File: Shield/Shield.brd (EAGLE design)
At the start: 100 x 80 mm, 11 parts, among them Q1 NPN, U1 TEMPERATURE-SENSOR

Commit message: fixed D2 pin
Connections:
- removed net D2: JP4.1
- net LED: now also JP4.1
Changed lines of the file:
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@@
 </elements>
 <signals>
-<signal name="D2">
-<contactref element="JP4" pad="1"/>
-</signal>
 <signal name="MST">
 <contactref element="YUN1" pad="A0"/>
@@
 <signal name="LED">
 <contactref element="YUN1" pad="D2"/>
+<contactref element="JP4" pad="1"/>
+<wire x1="53.312078125" y1="24.739640625" x2="26.27139375" y2="67.21223125" width="0" layer="19" extent="1-1"/>
 </signal>
 </signals>

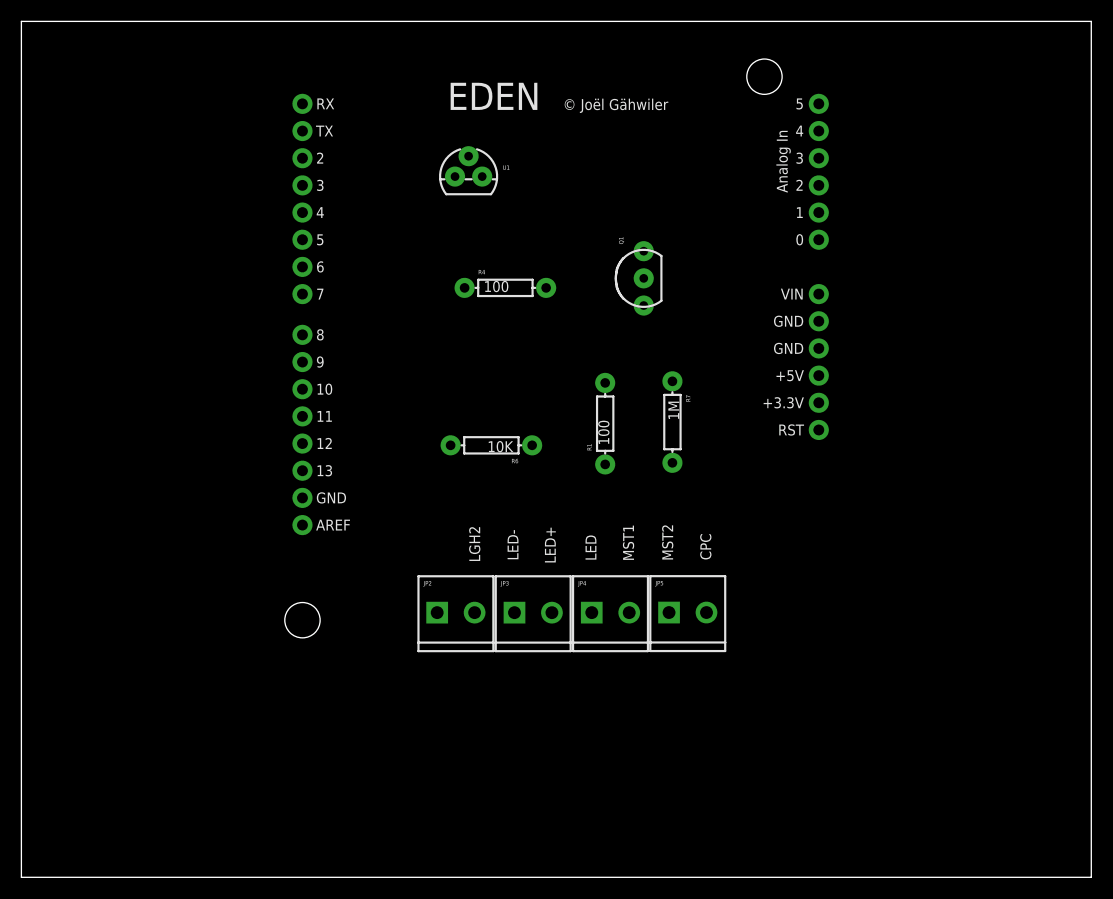
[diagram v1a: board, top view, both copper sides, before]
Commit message: finished shield v1.0
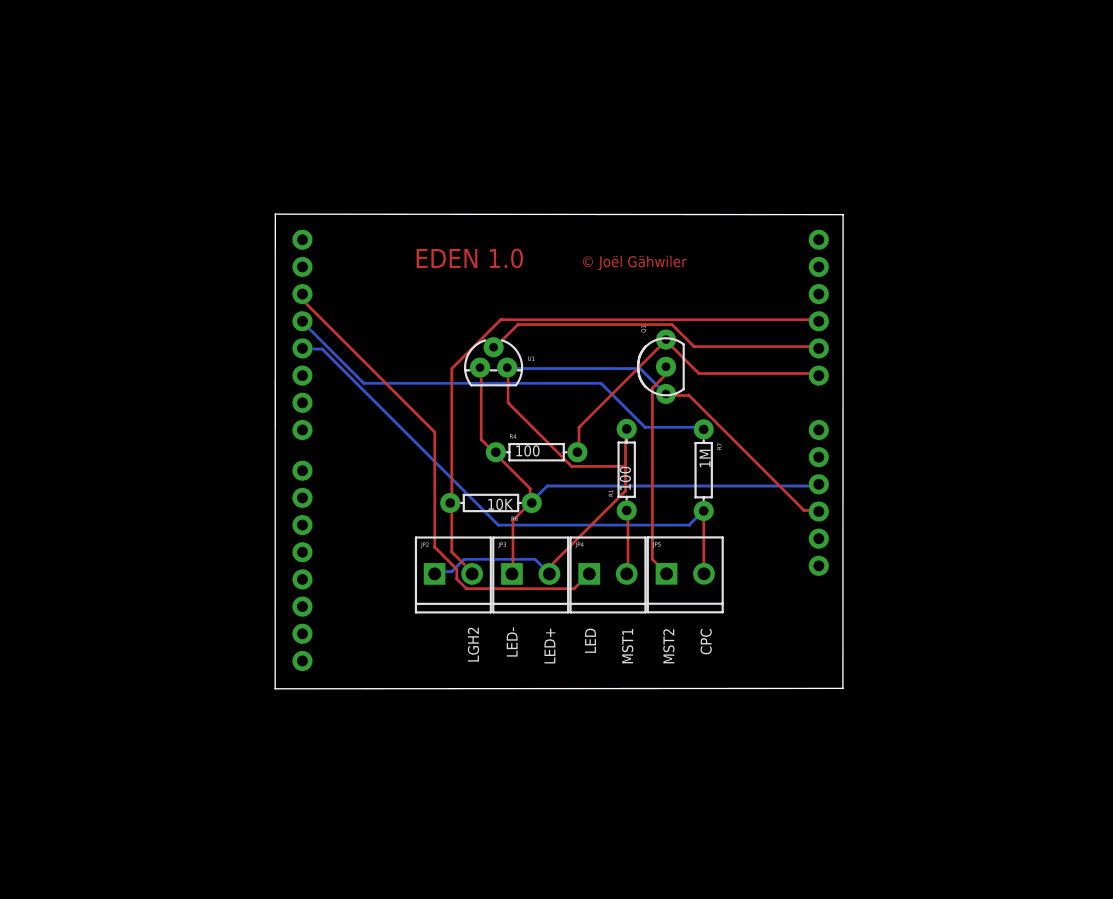
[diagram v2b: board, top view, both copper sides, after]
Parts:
- YUN1: device SparkFun-Boards:DUEMILANOVE_SHIELD -> SparkFun-Boards:DUEMILANOVE_VIAS
- moved U1 18.0 mm to (44.1, 47.6)
- moved R4 15.6 mm to (48.2, 39.7)
- moved Q1 8.52 mm to (60.3, 47.7)
- moved R6 5.39 mm to (43.9, 35.0)
- moved R7 5.36 mm to (63.8, 38.1)
- moved R1 4.75 mm to (56.6, 38.1)
- moved JP2 3.63 mm to (38.6, 28.4)
- moved JP3 3.63 mm to (45.9, 28.4)
- moved JP4 3.63 mm to (53.1, 28.4)
- moved JP5 3.63 mm to (60.3, 28.4)
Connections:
- net CAP1 renamed CPC1
- net CAP2 renamed CPC2
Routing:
- net VCC: track 0.00 -> 80.0 mm
- net LGH: track 0.00 -> 56.5 mm
- net CPC2: track 0.00 -> 50.8 mm
- net GND: track 0.00 -> 49.9 mm
- net LED: track 0.00 -> 45.9 mm
- net CPC1: track 0.00 -> 41.7 mm
- net TMP: track 0.00 -> 32.3 mm
- net MST: track 0.00 -> 29.8 mm
- net MST2: track 0.00 -> 20.4 mm
- net MST1: track 0.00 -> 5.98 mm
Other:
- board size 100 x 80 mm -> 53.1 x 44.4 mm
- board text added: "EDEN 1.0"
- board text removed: "EDEN"
